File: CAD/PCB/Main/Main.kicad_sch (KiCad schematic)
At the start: 55 parts, among them J1 GPIO, J2 XT60, J3 XT30, J4 JST_PH, J5 JST_PH, J6 JST_PH, J7 Conn_01x03, Q1 IAUC100N04S6N015ATMA1, U1 LMZ31707RVQR, U3 MCP3202T-CI/SN, U5 VNH5019ATR-E

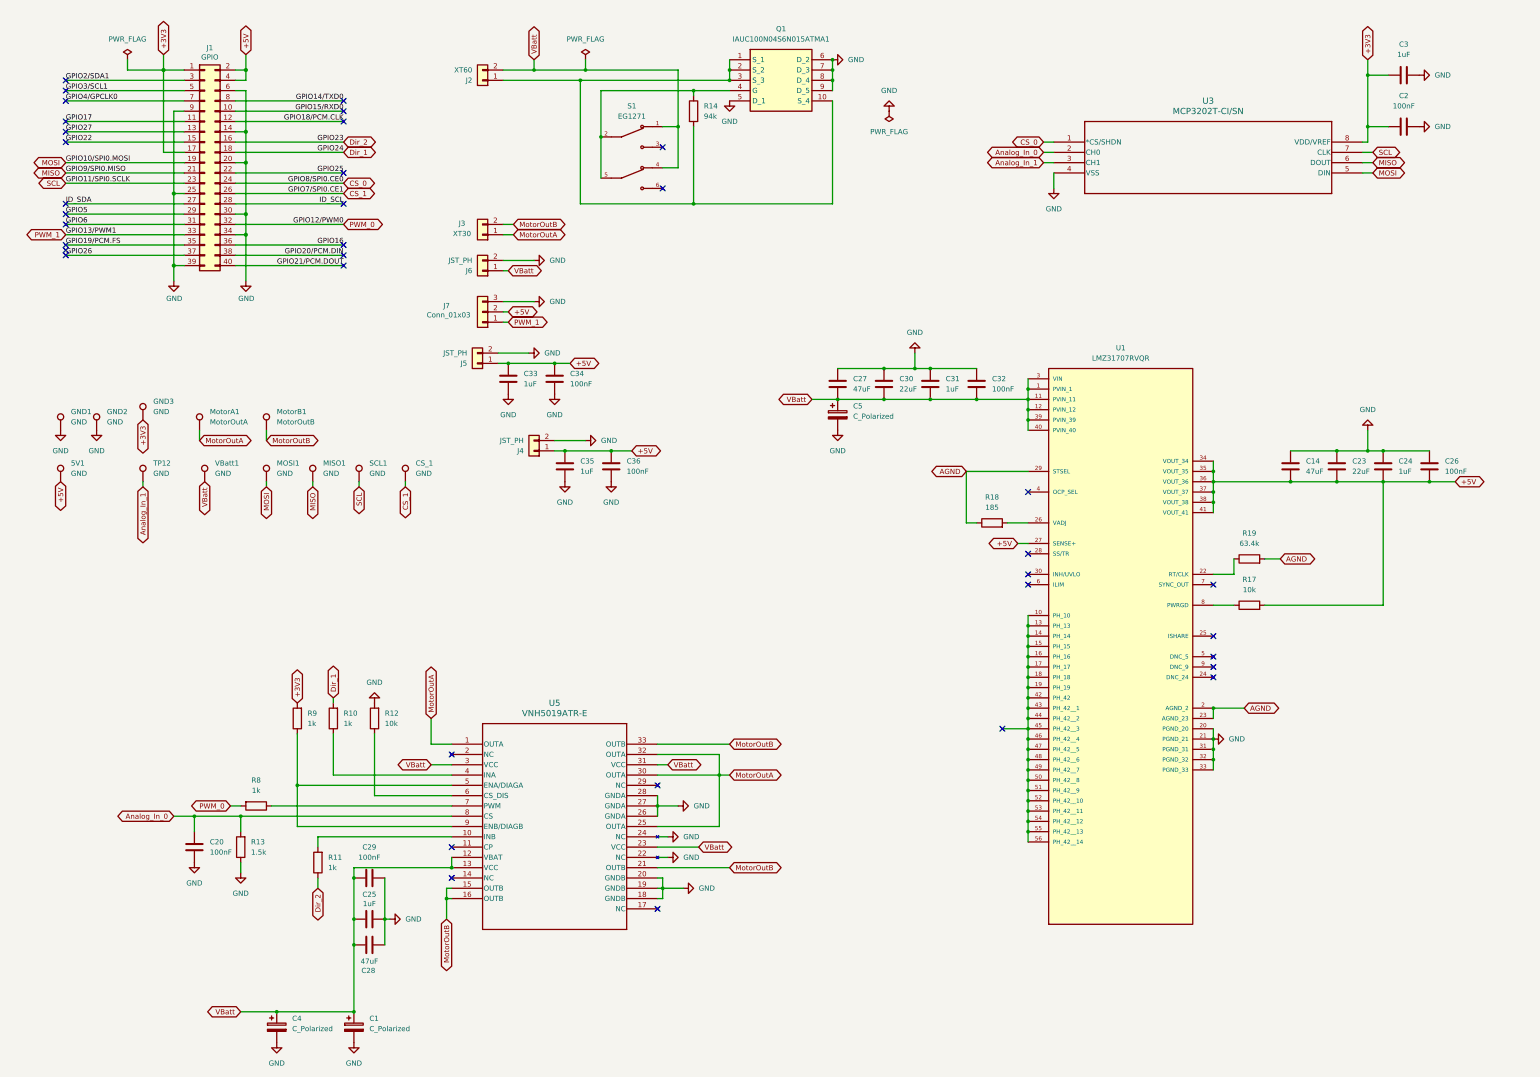
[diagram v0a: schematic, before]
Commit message: pcb order is in
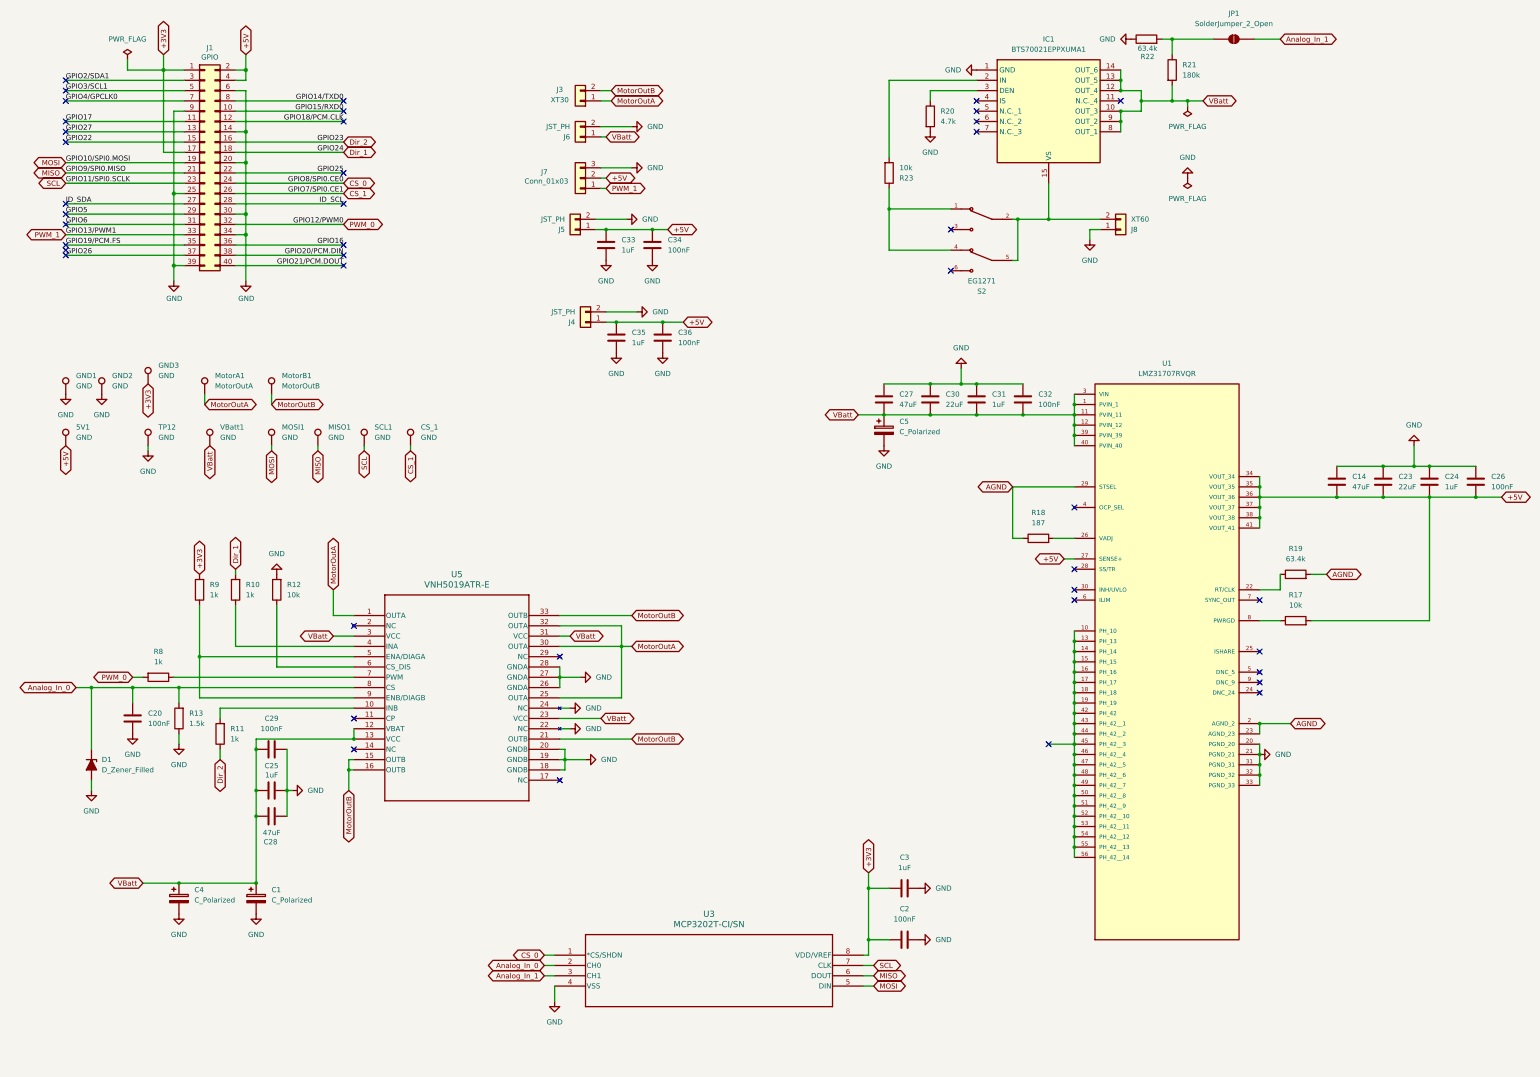
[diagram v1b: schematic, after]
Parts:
- removed J2: XT60, Connector_AMASS:AMASS_XT60-M_1x02_P7.20mm_Vertical, symbol Connector_Generic:Conn_01x02
- removed Q1: IAUC100N04S6N015ATMA1, RC_CAR:IPC100N04S51R2ATMA1, symbol RC_CAR:IAUC100N04S6N015ATMA1
- removed R14: 94k, Resistor_SMD:R_0805_2012Metric_Pad1.20x1.40mm_HandSolder, symbol Device:R
- removed S1: EG1271, RC_CAR:SW_EG1271, symbol RC_CAR:EG1271
- added D1: D_Zener_Filled, Diode_SMD:D_SOD-123F, symbol Device:D_Zener_Filled
- added IC1: BTS70021EPPXUMA1, RC_CAR:SOP65P600X115-15N, symbol RC_CAR:BTS70021EPPXUMA1
- added J8: XT60, Connector_AMASS:AMASS_XT60-M_1x02_P7.20mm_Vertical, symbol Connector_Generic:Conn_01x02
- added JP1: SolderJumper_2_Open, Jumper:SolderJumper-2_P1.3mm_Open_RoundedPad1.0x1.5mm, symbol Jumper:SolderJumper_2_Open
- added R20: 4.7k, Resistor_SMD:R_0805_2012Metric_Pad1.20x1.40mm_HandSolder, symbol Device:R
- added R21: 180k, Resistor_SMD:R_0805_2012Metric_Pad1.20x1.40mm_HandSolder, symbol Device:R
- added R22: 63.4k, Resistor_SMD:R_0805_2012Metric_Pad1.20x1.40mm_HandSolder, symbol Device:R
- added R23: 10k, Resistor_SMD:R_0805_2012Metric_Pad1.20x1.40mm_HandSolder, symbol Device:R
- added S2: EG1271, RC_CAR:SW_EG1271, symbol RC_CAR:EG1271
- R18: value 185 -> 187
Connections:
- net Analog_In_0: now also D1.1 (K)
- net Analog_In_1: now also JP1.2 (B); no longer TP12.1
- net GND: now also TP12.1, D1.2 (A), IC1.1 (GND), J8.1 (Pin_1), R20.2, R22.1
- net VBatt: now also IC1.10 (OUT_3), IC1.12 (OUT_4), IC1.13 (OUT_5), IC1.14 (OUT_6), IC1.8 (OUT_1), IC1.9 (OUT_2), R21.2
- new net: R23.1, S2.1, S2.4
- new net: IC1.2 (IN), R23.2
- new net: JP1.1 (A), R21.1, R22.2
- new net: IC1.15 (VS), J8.2 (Pin_2), S2.2, S2.5
- new net: IC1.3 (DEN), R20.1
- no-connect marks 37 -> 42
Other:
- moved on the sheet: 5V1, C1, C14, C2, C20, C23, C24, C25, C26, C27, C28, C29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
